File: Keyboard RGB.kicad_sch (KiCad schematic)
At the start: 31 parts, among them J2 OLED_128x64, U2 Arduino_Pro_Micro

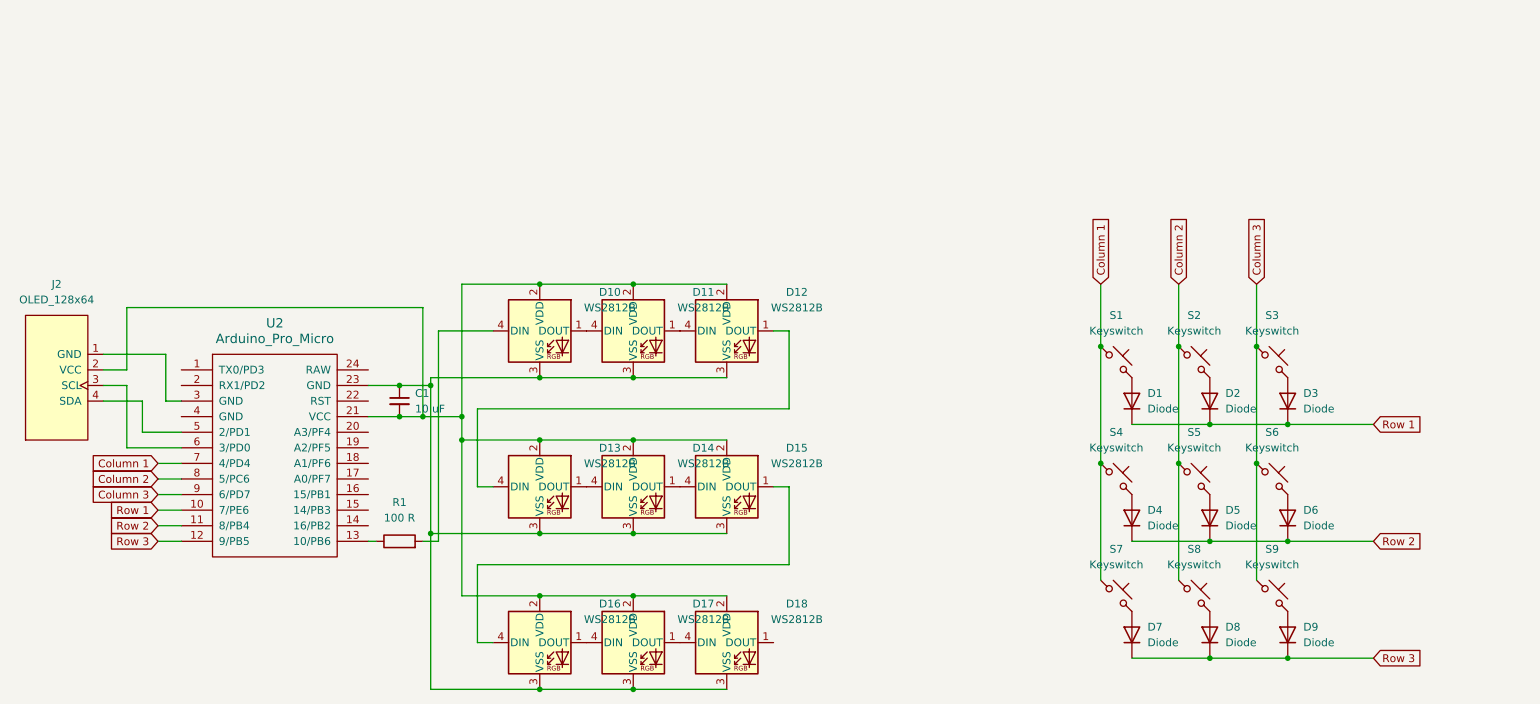
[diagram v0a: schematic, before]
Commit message: updated schematic
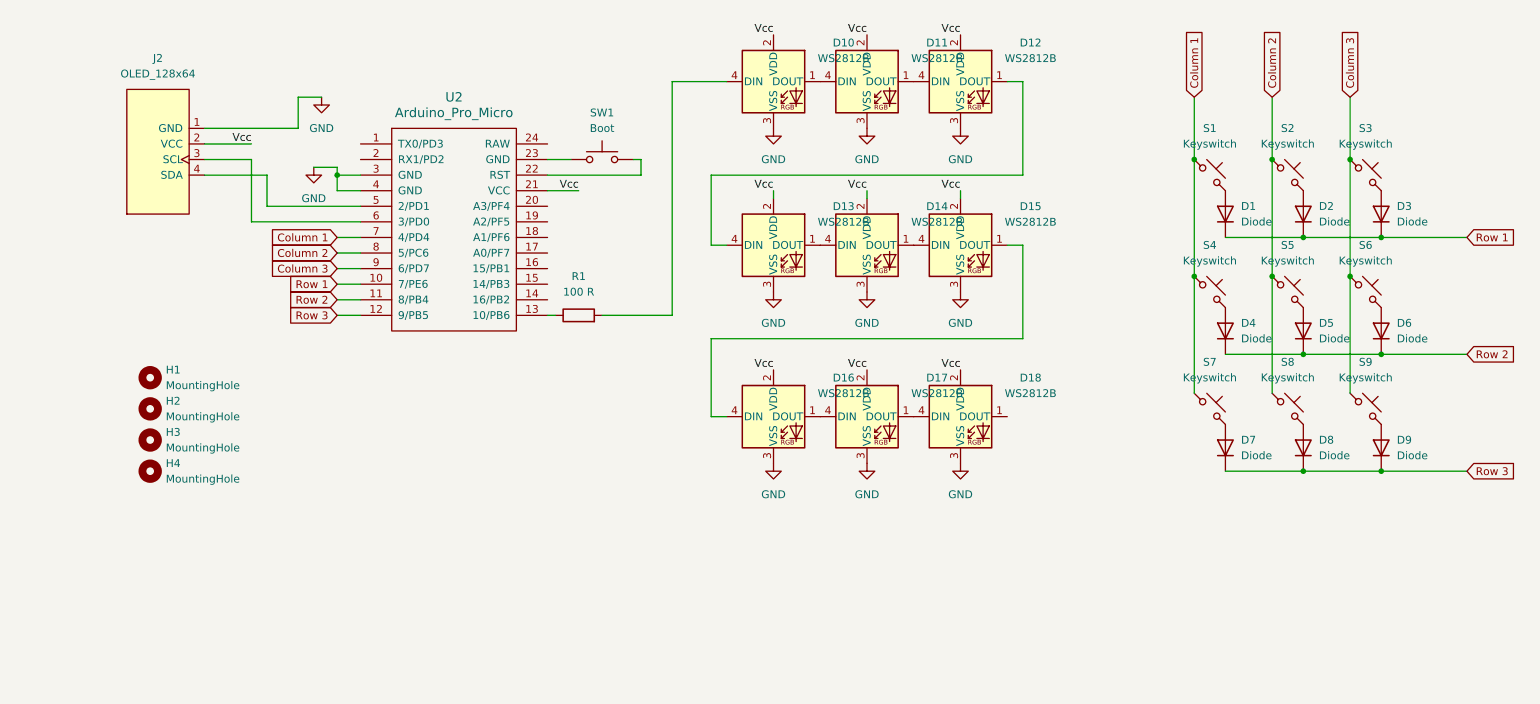
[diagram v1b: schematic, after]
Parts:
- removed C1: 10 uF, Capacitor_SMD:C_0805_2012Metric, symbol Device:C_Small
- added H1, H2, H3, H4: MountingHole, MountingHole:MountingHole_3.2mm_M3_DIN965_Pad, symbol Mechanical:MountingHole
- added SW1: Boot, Button_Switch_THT:SW_PUSH_6mm_H4.3mm, symbol Switch:SW_Push
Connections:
- net Vcc: now reaches D10.2 (VDD), D11.2 (VDD), D12.2 (VDD), D13.2 (VDD), D14.2 (VDD), D15.2 (VDD), D16.2 (VDD), D17.2 (VDD), D18.2 (VDD), J2.2 (VCC), U2.21 (VCC)
- net GND: now reaches D10.3 (VSS), D11.3 (VSS), D12.3 (VSS), D13.3 (VSS), D14.3 (VSS), D15.3 (VSS), D16.3 (VSS), D17.3 (VSS), D18.3 (VSS)
- net GND: now also J2.1 (GND), U2.3 (GND), U2.4 (GND); no longer U2.23 (GND)
- net at U2.22 (RST): now also SW1.2
- new net: SW1.1, U2.23 (GND)
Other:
- moved on the sheet: D1, D10, D11, D12, D13, D14, D15, D16, D17, D18, D2, D3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

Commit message: cleaned schematic, updated traces, components and zones
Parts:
- J2: footprint ScottoKeebs_Components:OLED_128x64 -> Connector_JST:JST_EH_B4B-EH-A_1x04_P2.50mm_Vertical
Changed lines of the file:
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@@
 			)
 		)
-		(property "Footprint" "ScottoKeebs_Components:OLED_128x64"
+		(property "Footprint" "Connector_JST:JST_EH_B4B-EH-A_1x04_P2.50mm_Vertical"
 			(at 30.48 64.77 0)
 			(effects
